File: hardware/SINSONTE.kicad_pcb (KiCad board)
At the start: 2 copper layers, 90 x 70 mm, 35 parts, among them J1 BAT, J10 Conn_01x01_Male, J11 Conn_01x01_Male, J12 Conn_01x04_Male, J13 Conn_01x01_Male, J14 Conn_01x02_Male, J2 CLOCK, J3 LIGHT_SENSOR, J4 Conn_01x17_Male, J5 Conn_01x01_Male, J6 Conn_01x01_Male, J7 Conn_01x01_Male, J8 Conn_01x01_Male, J9 PROG, Q1 2N7000, Q2 PN2222A, SW1 SW_Push, U1 Pico

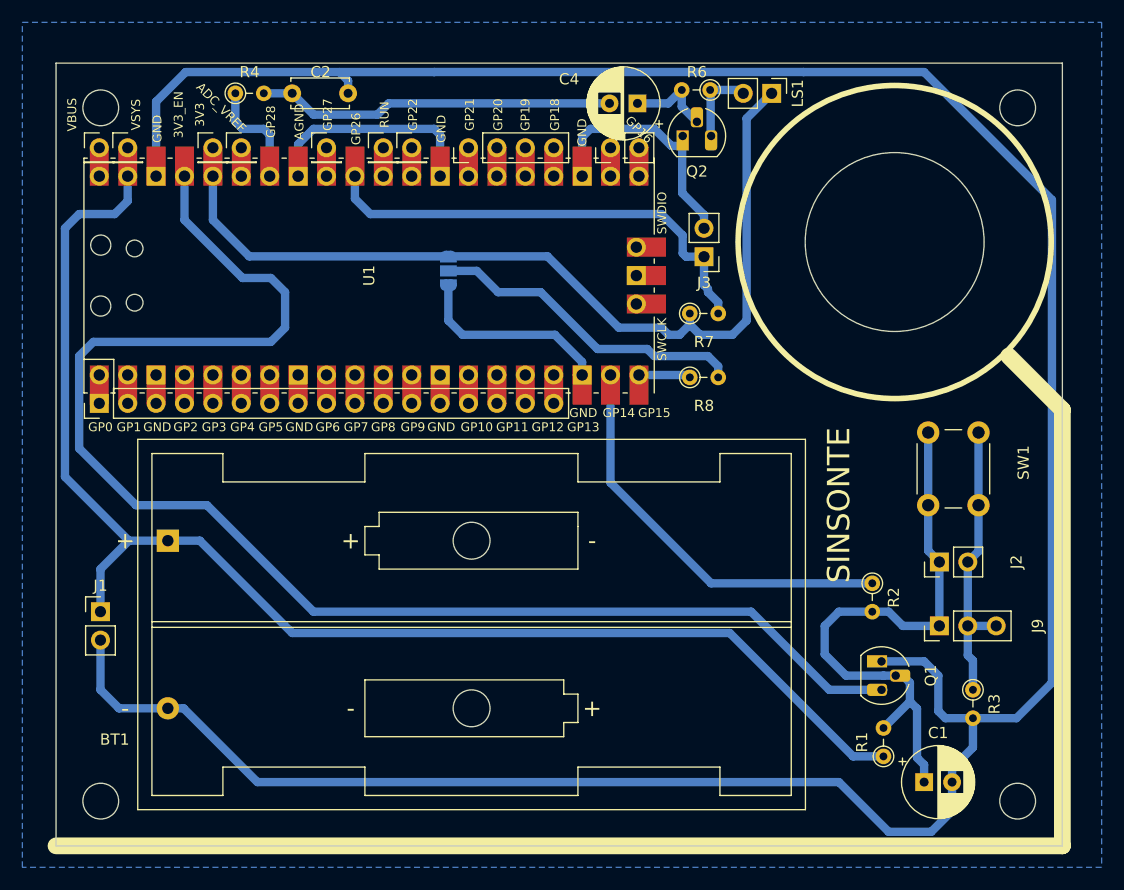
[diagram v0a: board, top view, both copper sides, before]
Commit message: top silks finished
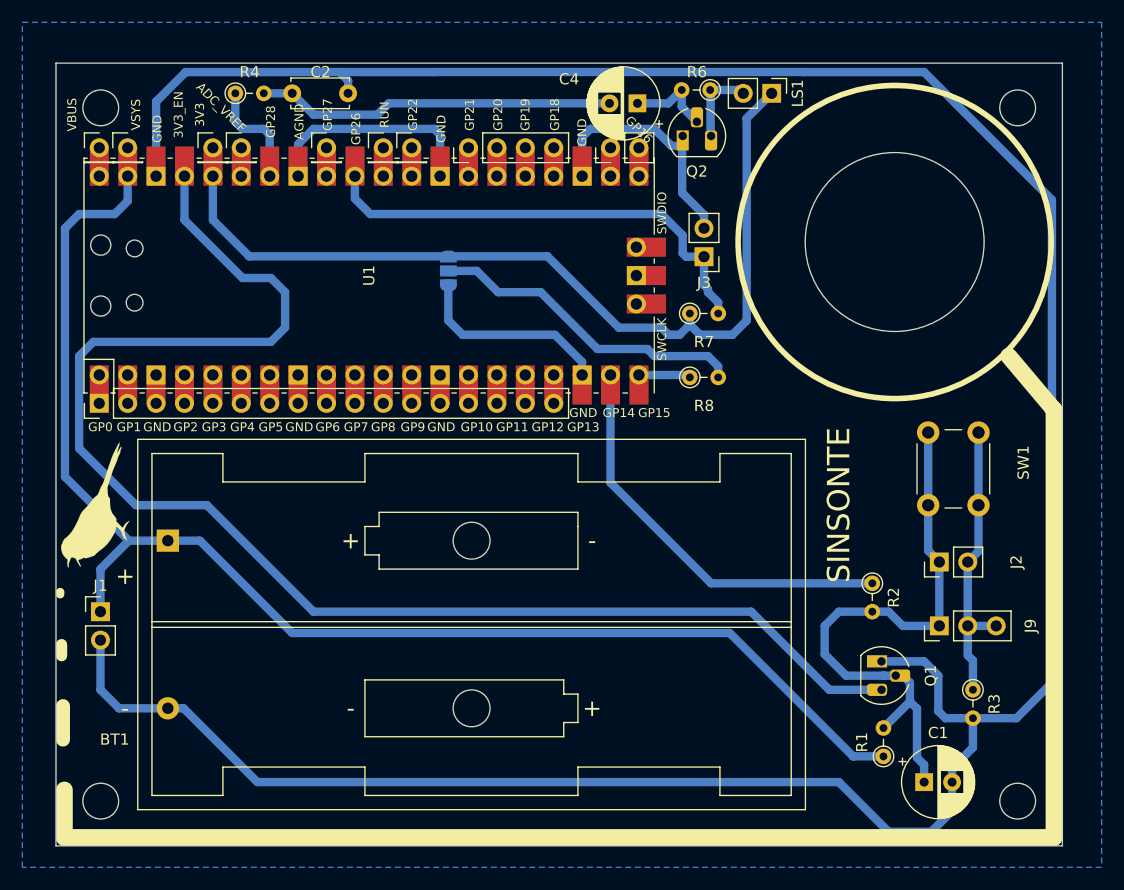
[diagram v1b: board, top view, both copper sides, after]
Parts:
- added G***: LOGO, Logos_Galopago:sinsonte_logo_11x6mm, F.Cu at (53.5, 89.5)
